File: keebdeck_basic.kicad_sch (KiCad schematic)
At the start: 108 parts, among them J1 USB_C_Receptacle_USB2.0, J2 Conn_Qwiic, SW1 SW_ESC, SW10 SW_1, SW11 SW_2, SW12 SW_3, SW13 SW_4, SW14 SW_5, SW15 SW_6, SW16 SW_7, SW17 SW_8, SW18 SW_9, SW19 SW_0, SW2 SW_SQUARE, SW20 SW_-, SW21 SW_=, SW22 SW_TAB, SW23 SW_Q, SW24 SW_W, SW25 SW_E, SW26 SW_R, SW27 SW_T, SW28 SW_Y, SW29 SW_U, SW3 SW_TRIANGLE, SW30 SW_I, SW31 SW_O, SW32 SW_P, SW33 SW_[, SW34 SW_], SW35 SW_FN, SW36 SW_A, SW37 SW_S, SW38 SW_D, SW39 SW_F, SW4 SW_CROSS, SW40 SW_G, SW41 SW_H, SW42 SW_J, SW43 SW_K, SW44 SW_L, SW45 SW_;, SW46 SW_', SW47 SW_ENTER, SW48 SW_LSHIFT, SW49 SW_Z, SW5 SW_CIRCLE, SW50 SW_X, SW51 SW_C, SW52 SW_V, SW53 SW_B, SW54 SW_N, SW55 SW_M, SW56 SW_,, SW57 SW_., SW58 SW_/, SW59 SW_UP, SW6 SW_CLUB, SW60 SW_RSHIFT, SW61 SW_CTRL, SW62 SW_SP, SW63 SW_LALT, SW64 SW_\, SW65 SW_SPACE1, SW66 SW_SPACE2, SW67 SW_SPACE3, SW68 SW_RALT, SW69 SW_LEFT, SW7 SW_DIAMOND, SW70 SW_DOWN, SW71 SW_RIGHT, SW72 SW_BOOT, SW8 SW_BACKSPACE, SW9 SW_TILDE, U1 AP3032KTR, U2 AP2112K-3.3, U3 STM32F042G6Ux

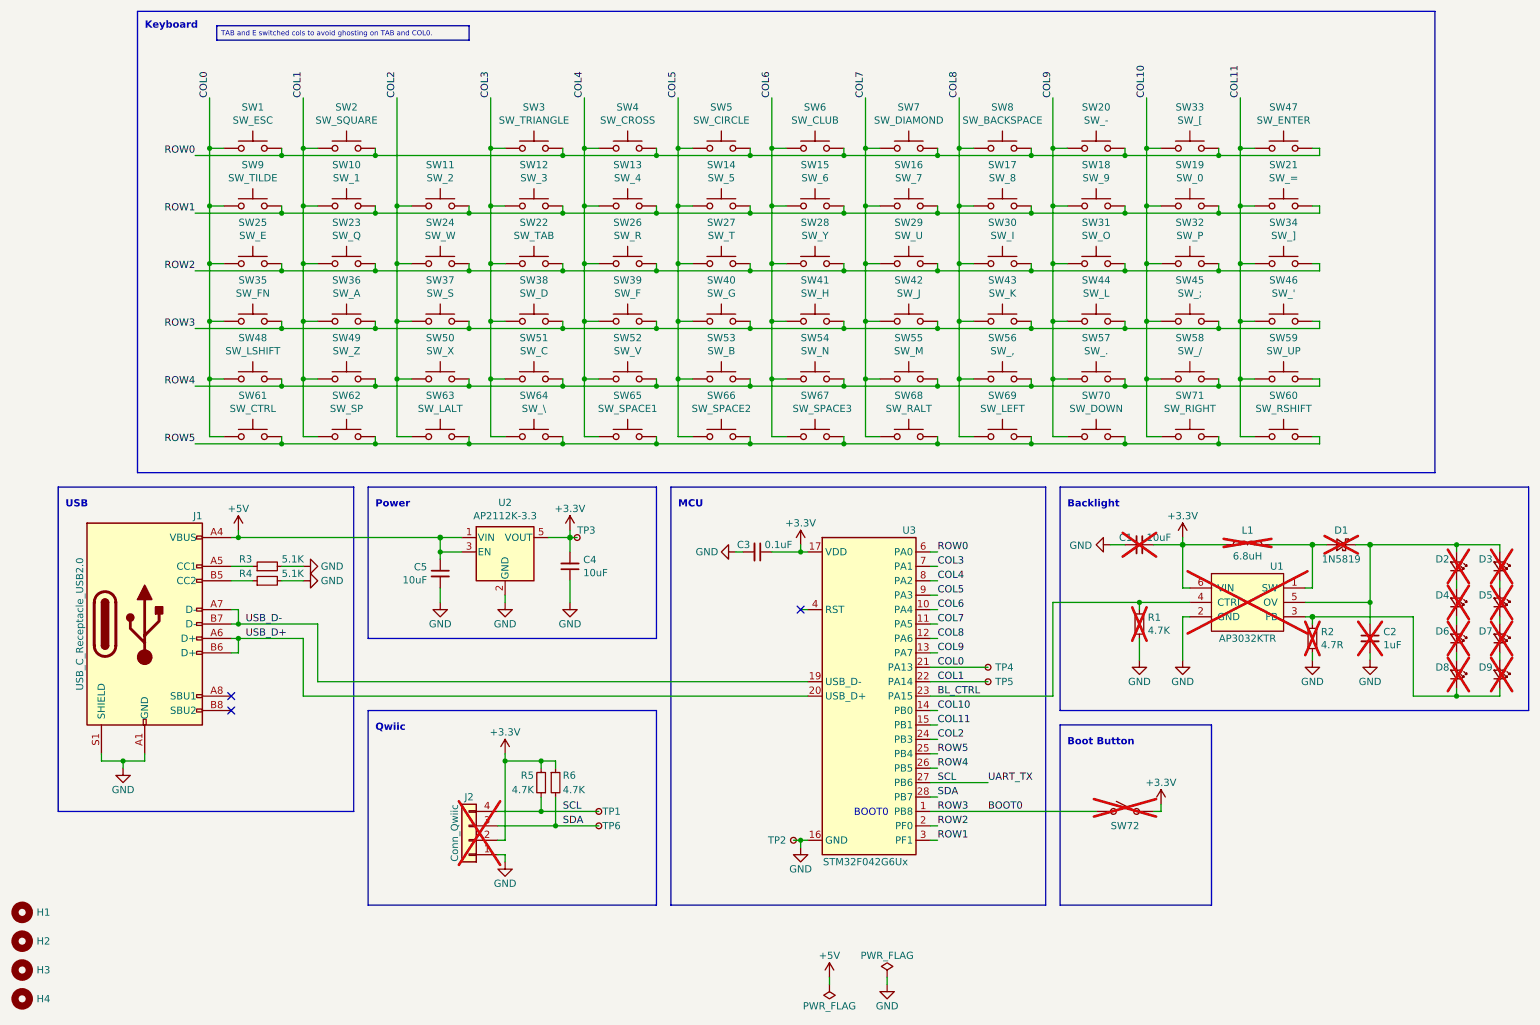
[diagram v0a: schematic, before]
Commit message: Rev 1.1 - Production
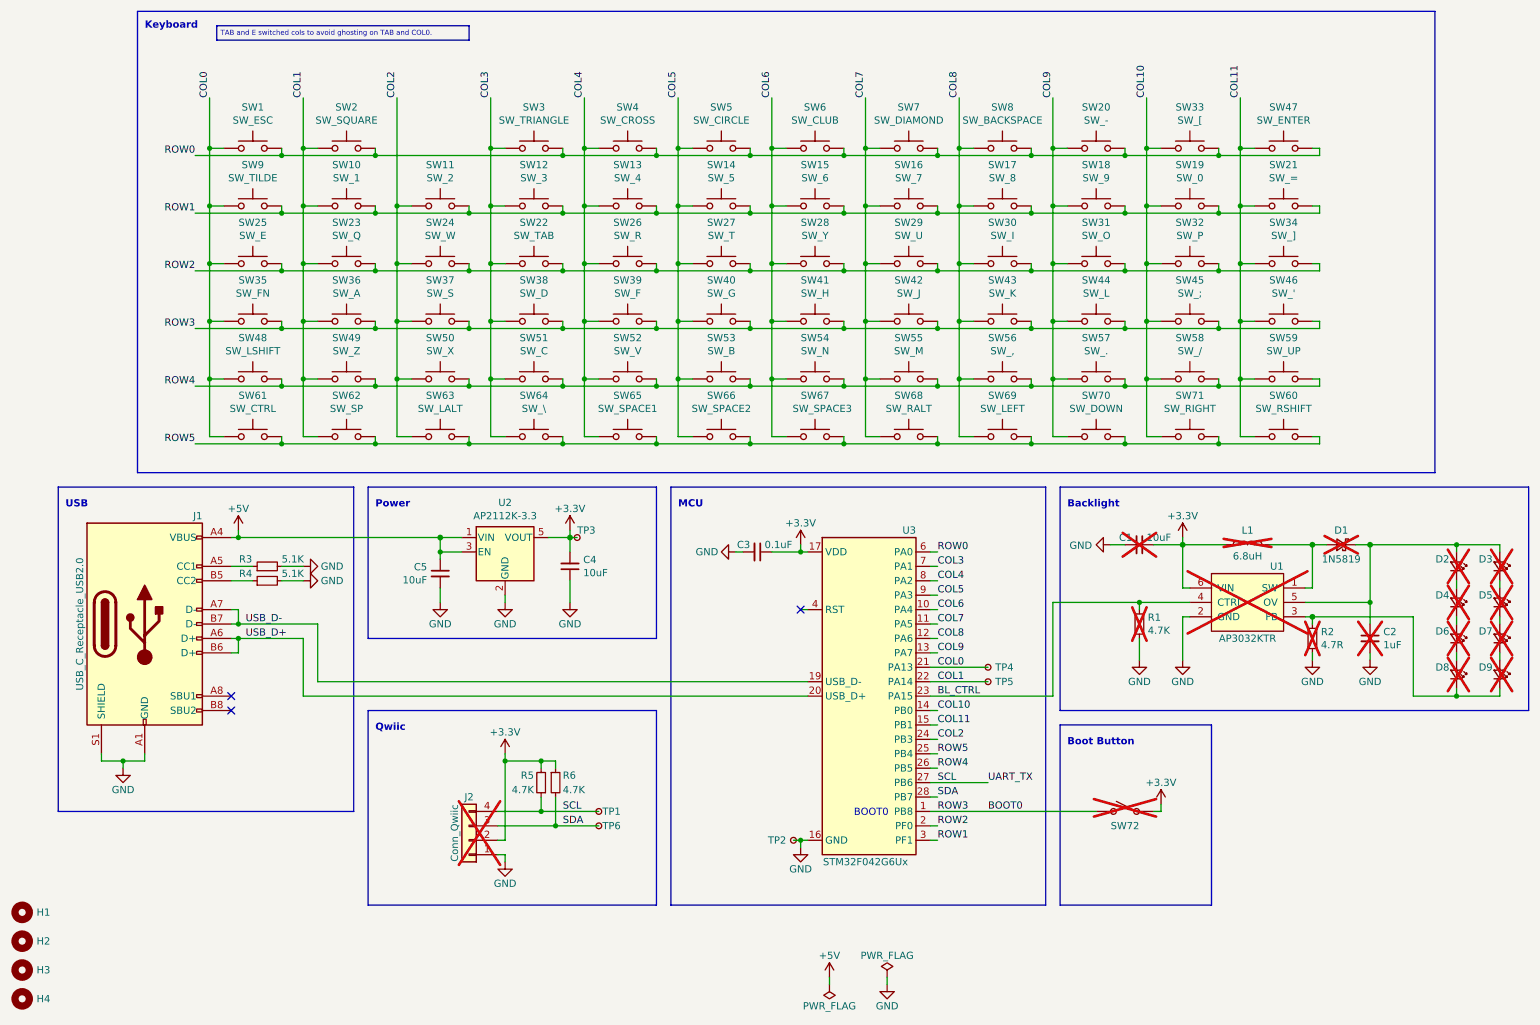
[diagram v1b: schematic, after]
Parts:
- U3: LCSC C2971720 -> C961597
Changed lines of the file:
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@@
 (kicad_sch
-	(version 20231120)
+	(version 20250114)
 	(generator "eeschema")
-	(generator_version "8.0")
+	(generator_version "9.0")
 	(paper "A4")
+	(rectangle
+		(start 77.47 142.24)
+		(end 128.27 176.53)
+		(stroke
+			(width 0)
+			(type default)
+		)
+		(fill
+			(type none)
+		)
+	)
+	(rectangle
+		(start 77.47 102.87)
+		(end 128.27 129.54)
+		(stroke
+			(width 0)
+			(type default)
+		)
+		(fill
+			(type none)
+		)
+	)
+	(rectangle
+		(start 130.81 102.87)
+		(end 196.85 176.53)
+		(stroke
+			(width 0)
+			(type default)
+		)
+		(fill
+			(type none)
+		)
+	)
+	(rectangle
+		(start 36.83 19.05)
+		(end 265.43 100.33)
+		(stroke
+			(width 0)
+			(type default)
+		)
+		(fill
+			(type none)
+		)
+	)
+	(rectangle
+		(start 22.86 102.87)
+		(end 74.93 160.02)
+		(stroke
+			(width 0)
+			(type default)
+		)
+		(fill
+			(type none)
+		)
+	)
+	(rectangle
+		(start 199.39 102.87)
+		(end 281.94 142.24)
+		(stroke
+			(width 0)
+			(type default)
+		)
+		(fill
+			(type none)
+		)
+	)
+	(rectangle
+		(start 199.39 144.78)
+		(end 226.06 176.53)
+		(stroke
+			(width 0)
+			(type default)
+		)
+		(fill
+			(type none)
+		)
+	)
+	(text "Keyboard"
+		(exclude_from_sim no)
+		(at 38.1 21.59 0)
+		(effects
+			(font
+				(size 1.27 1.27)
+				(thickness 0.254)
+				(bold yes)
+			)
+			(justify left)
+		)
+	)
+	(text "Boot Button"
+		(exclude_from_sim no)
+		(at 200.66 148.59 0)
+		(effects
+			(font
+				(size 1.27 1.27)
+				(thickness 0.254)
+				(bold yes)
+			)
+			(justify left bottom)
+		)
+	)
+	(text "USB"
+		(exclude_from_sim no)
+		(at 24.13 106.68 0)
+		(effects
+			(font
+				(size 1.27 1.27)
+				(thickness 0.254)
+				(bold yes)
+			)
+			(justify left bottom)
+		)
+	)
+	(text "Backlight"
+		(exclude_from_sim no)
+		(at 200.66 106.68 0)
+		(effects
+			(font
+				(size 1.27 1.27)
+				(thickness 0.254)
+				(bold yes)
+			)
+			(justify left bottom)
+		)
+	)
+	(text "Qwiic"
+		(exclude_from_sim no)
+		(at 78.74 146.05 0)
+		(effects
+			(font
+				(size 1.27 1.27)
+				(thickness 0.254)
+				(bold yes)
+			)
+			(justify left bottom)
+		)
+	)
+	(text "BOOT0"
+		(exclude_from_sim no)
+		(at 169.164 161.036 0)
+		(effects
+			(font
+				(size 1.27 1.27)
+			)
+			(justify right bottom)
+		)
+	)
+	(text "MCU\n"
+		(exclude_from_sim no)
+		(at 132.08 106.68 0)
+		(effects
+			(font
+				(size 1.27 1.27)
+				(thickness 0.254)
+				(bold yes)
+			)
+			(justify left bottom)
+		)
+	)
+	(text "Power"
+		(exclude_from_sim no)
+		(at 78.74 106.68 0)
+		(effects
+			(font
+				(size 1.27 1.27)
+				(thickness 0.254)
+				(bold yes)
+			)
+			(justify left bottom)
+		)
+	)
+	(text_box "TAB and E switched cols to avoid ghosting on TAB and COL0."
+		(exclude_from_sim no)
+		(at 50.8 21.59 0)
+		(size 44.45 2.54)
+		(margins 0.6668 0.6668 0.6668 0.6668)
+		(stroke
+			(width 0)
+			(type default)
+			(color 204 102 0 1)
+		)
+		(fill
+			(type color)
+			(color 255 255 194 1)
+		)
+		(effects
+			(font
+				(size 0.889 0.889)
+				(color 204 102 0 1)
+			)
+			(justify left top)
+		)
+	)
 	(junction
 		(at 210.82 64.77)
@@
 		)
 	)
-	(rectangle
-		(start 77.47 142.24)
-		(end 128.27 176.53)
-		(stroke
-			(width 0)
-			(type default)
-		)
-		(fill
-			(type none)
-		)
-	)
-	(rectangle
-		(start 77.47 102.87)
-		(end 128.27 129.54)
-		(stroke
-			(width 0)
-			(type default)
-		)
-		(fill
-			(type none)
-		)
-	)
-	(rectangle
-		(start 130.81 102.87)
-		(end 196.85 176.53)
-		(stroke
-			(width 0)
-			(type default)
-		)
-		(fill
-			(type none)
-		)
-	)
-	(rectangle
-		(start 36.83 19.05)
-		(end 265.43 100.33)
-		(stroke
-			(width 0)
-			(type default)
-		)
-		(fill
-			(type none)
-		)
-	)
-	(rectangle
-		(start 22.86 102.87)
-		(end 74.93 160.02)
-		(stroke
-			(width 0)
-			(type default)
-		)
-		(fill
-			(type none)
-		)
-	)
-	(rectangle
-		(start 199.39 102.87)
-		(end 281.94 142.24)
-		(stroke
-			(width 0)
-			(type default)
-		)
-		(fill
-			(type none)
-		)
-	)
-	(rectangle
-		(start 199.39 144.78)
-		(end 226.06 176.53)
-		(stroke
-			(width 0)
-			(type default)
-		)
-		(fill
-			(type none)
-		)
-	)
-	(text_box "TAB and E switched cols to avoid ghosting on TAB and COL0."
-		(exclude_from_sim no)
-		(at 50.8 21.59 0)
-		(size 44.45 2.54)
-		(stroke
-			(width 0)
-			(type default)
-			(color 204 102 0 1)
-		)
-		(fill
-			(type color)
-			(color 255 255 194 1)
-		)
-		(effects
-			(font
-				(size 0.889 0.889)
-				(color 204 102 0 1)
-			)
-			(justify left top)
-		)
-	)
-	(text "Keyboard"
-		(exclude_from_sim no)
-		(at 38.1 21.59 0)
-		(effects
-			(font
-				(size 1.27 1.27)
-				(thickness 0.254)
-				(bold yes)
-			)
-			(justify left)
-		)
-	)
-	(text "Boot Button"
-		(exclude_from_sim no)
-		(at 200.66 148.59 0)
-		(effects
-			(font
-				(size 1.27 1.27)
-				(thickness 0.254)
-				(bold yes)
-			)
-			(justify left bottom)
-		)
-	)
-	(text "USB"
-		(exclude_from_sim no)
-		(at 24.13 106.68 0)
-		(effects
-			(font
-				(size 1.27 1.27)
-				(thickness 0.254)
-				(bold yes)
-			)
-			(justify left bottom)
-		)
-	)
-	(text "Backlight"
-		(exclude_from_sim no)
-		(at 200.66 106.68 0)
-		(effects
-			(font
-				(size 1.27 1.27)
-				(thickness 0.254)
-				(bold yes)
-			)
-			(justify left bottom)
-		)
-	)
-	(text "Qwiic"
-		(exclude_from_sim no)
-		(at 78.74 146.05 0)
-		(effects
-			(font
-				(size 1.27 1.27)
-				(thickness 0.254)
-				(bold yes)
-			)
-			(justify left bottom)
-		)
-	)
-	(text "BOOT0"
-		(exclude_from_sim no)
-		(at 169.164 161.036 0)
-		(effects
-			(font
-				(size 1.27 1.27)
-			)
-			(justify right bottom)
-		)
-	)
-	(text "MCU\n"
-		(exclude_from_sim no)
-		(at 132.08 106.68 0)
-		(effects
-			(font
-				(size 1.27 1.27)
-				(thickness 0.254)
-				(bold yes)
-			)
-			(justify left bottom)
-		)
-	)
-	(text "Power"
-		(exclude_from_sim no)
-		(at 78.74 106.68 0)
-		(effects
-			(font
-				(size 1.27 1.27)
-				(thickness 0.254)
-				(bold yes)
-			)
-			(justify left bottom)
-		)
-	)
 	(label "COL3"
 		(at 177.8 116.84 0)
@@
 			)
 		)
-		(property "LCSC" "C2971720"
+		(property "LCSC" "C961597"
 			(at 165.1 139.7 0)
 			(effects
@@
 		)
 	)
+	(embedded_fonts no)
 )
